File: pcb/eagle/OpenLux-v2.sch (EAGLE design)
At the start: 81 parts, among them IC1 MCP73871, IC2 ATMEGA32U4-AU, U1 USD-SOCKETMICRO-SD-SOCKET-TAO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, U2 XBEE, U3 MLX90614_, X1 8MHz

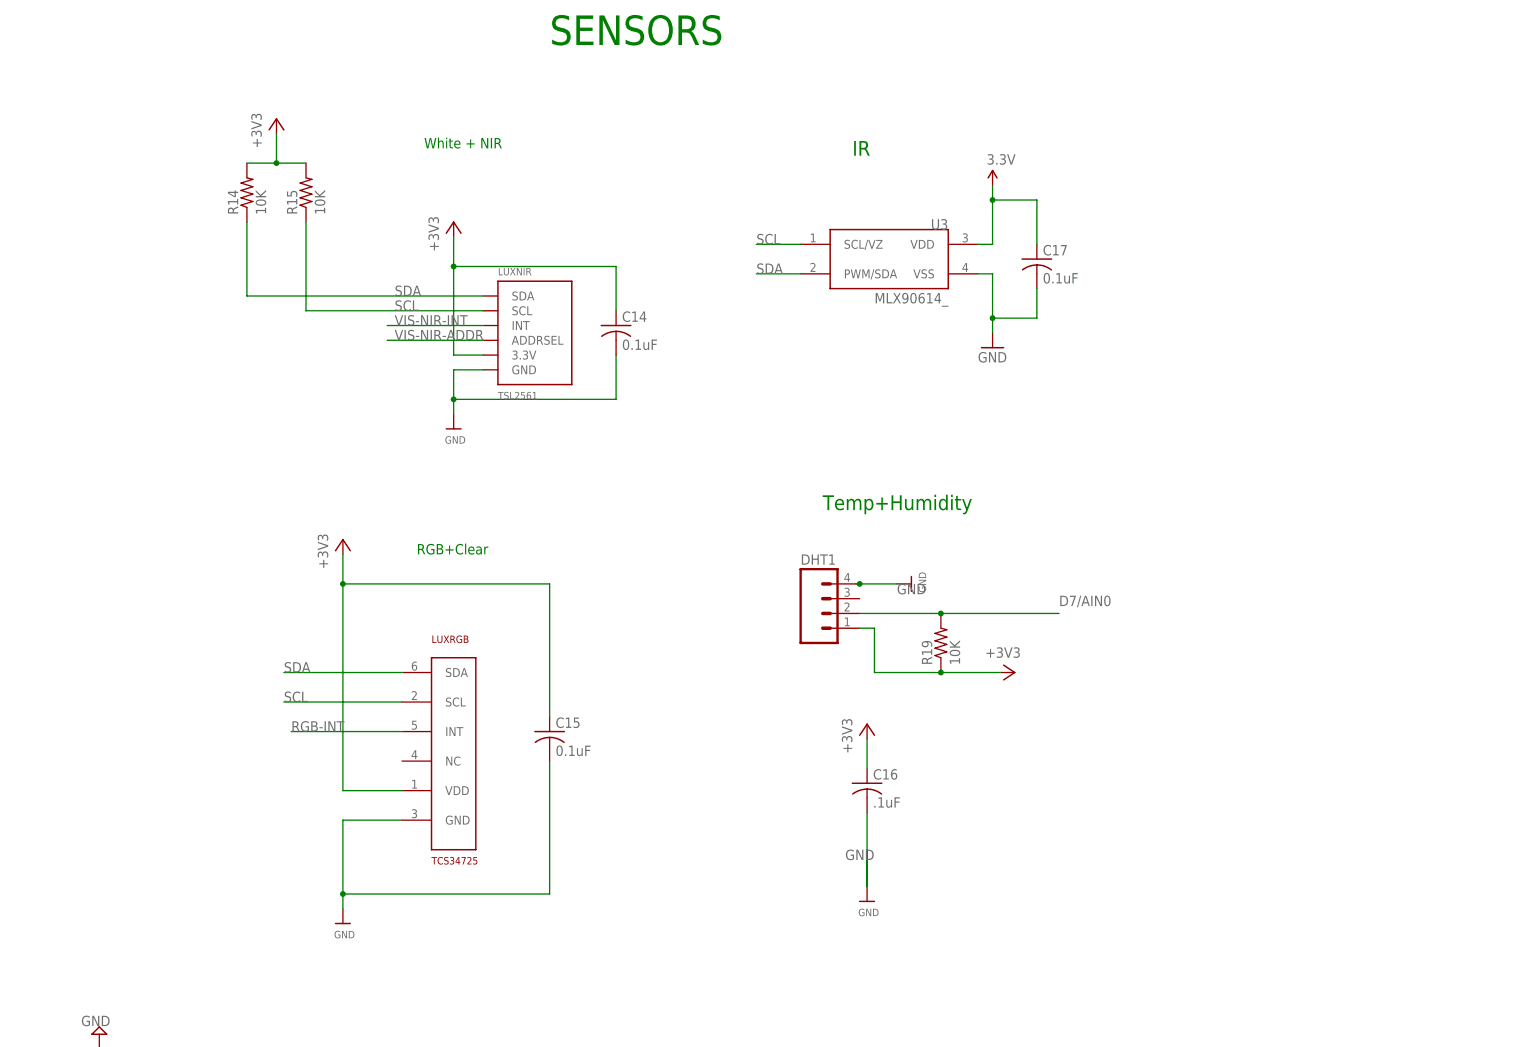
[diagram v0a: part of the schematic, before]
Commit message: added some schematics
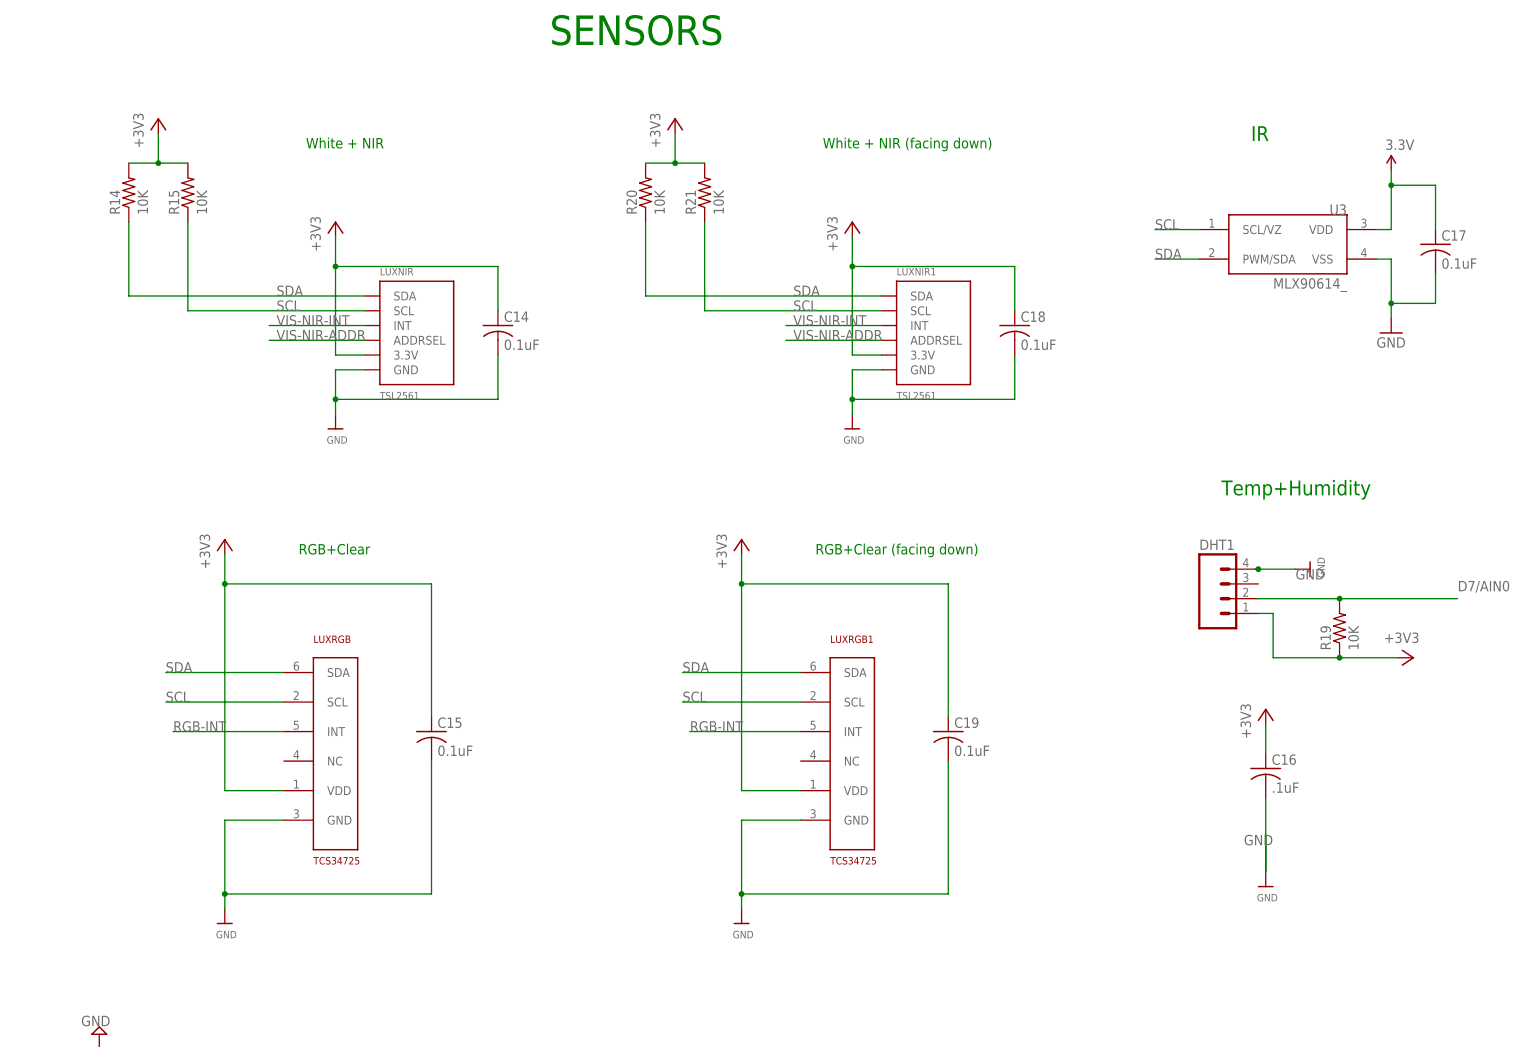
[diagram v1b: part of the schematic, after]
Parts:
- added C18, C19: 0.1uF, adafruit:C-USC0805
- added LUXNIR1: TSL2561, microbuilder:TSL2561
- added LUXRGB1: TCS34725, dwbLibrary:TCS34725
- added R20, R21: 10K, adafruit:R-US_R0805
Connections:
- net +3V3: now also C18.1, C19.1, LUXNIR1.3.3V, LUXRGB1.VDD, R20.2, R21.2
- net GND: now also C18.2, C19.2, LUXNIR1.GND, LUXRGB1.GND
- net RGB-INT: now also LUXRGB1.INT
- net SCL: now also LUXNIR1.SCL, LUXRGB1.SCL, R21.1
- net SDA: now also LUXNIR1.SDA, LUXRGB1.SDA, R20.1
- net VIS-NIR-ADDR: now also LUXNIR1.ADDRSEL
- net VIS-NIR-INT: now also LUXNIR1.INT
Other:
- note added: "RGB+Clear (facing down)"
- note added: "White + NIR (facing down)"
- moved on the sheet: C14, C15, C16, C17, DHT1, LUXNIR, LUXRGB, R14, R15, R19, U3
